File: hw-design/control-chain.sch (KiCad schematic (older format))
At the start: 25 parts, among them J1 RJ45_CHAIN_MAIN, J2 RJ45_CHAIN_EXTENSION, Q1 MMBT3904, Q2 MMBT3906, U4 MAX13450E

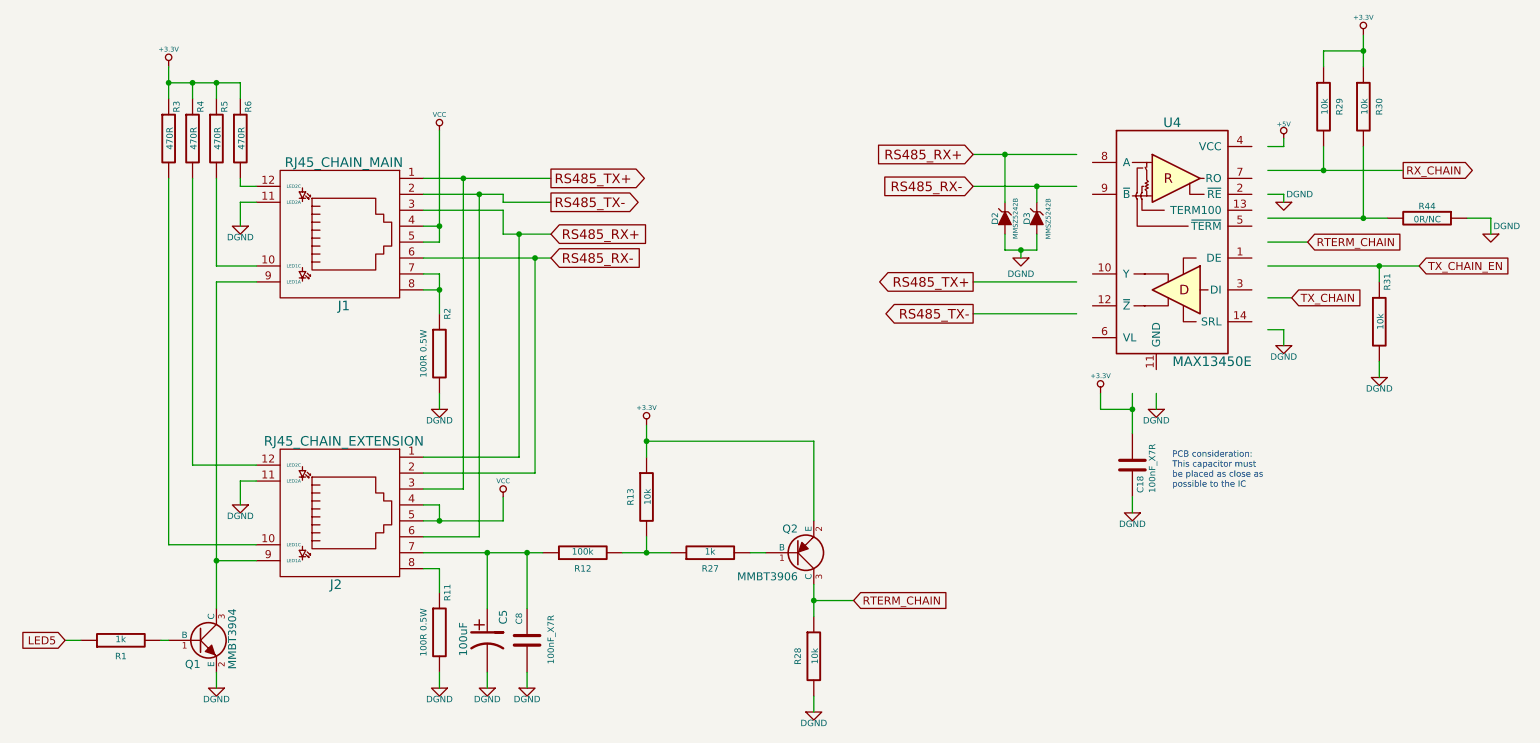
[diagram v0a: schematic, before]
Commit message: updating MAX13450E symbol
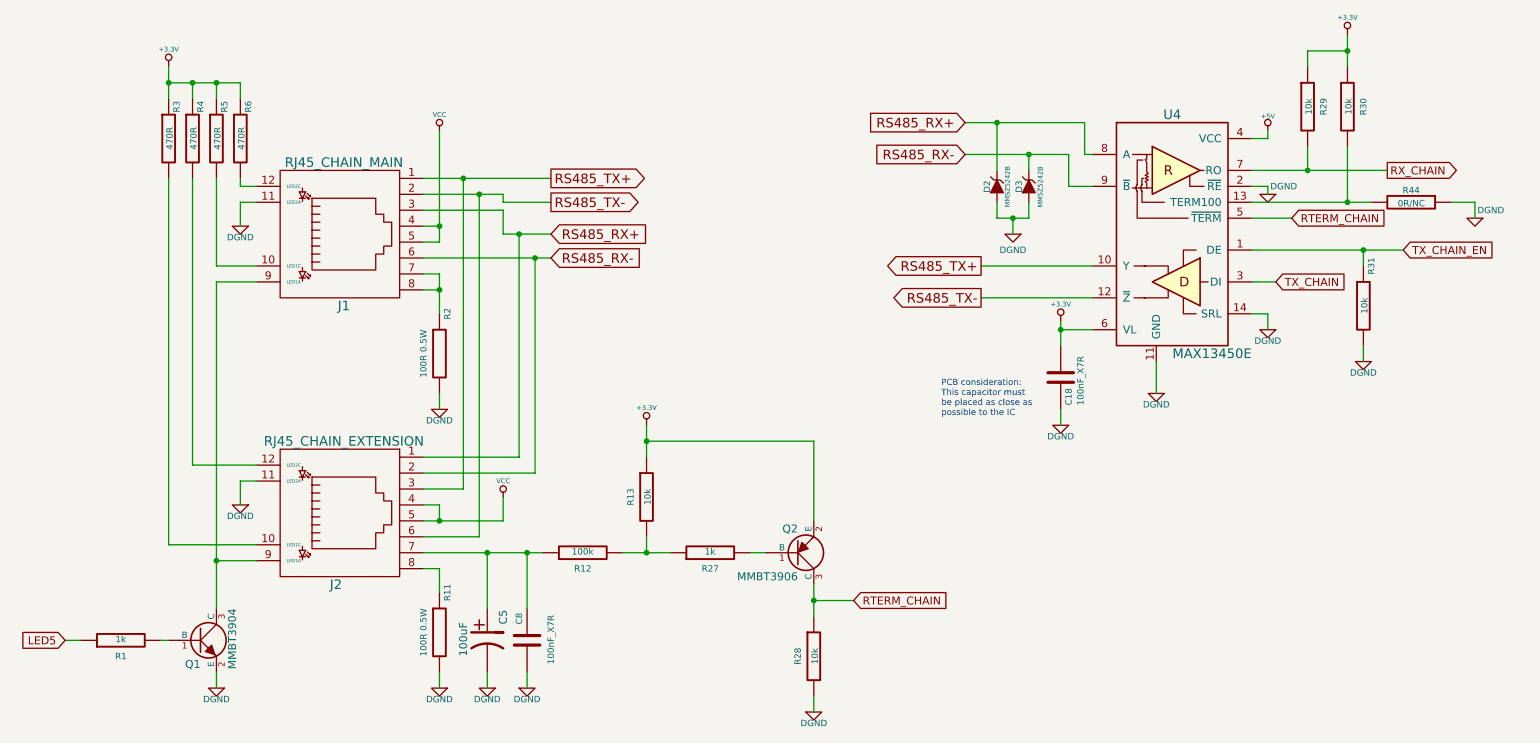
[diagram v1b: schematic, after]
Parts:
- U4: footprint MOD_Footprints_Lib:TSSOP14 -> TSSOP-14EP
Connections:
- wire segments 102 -> 105
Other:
- moved on the sheet: C18, D2, D3, R29, R30, R31, R44
